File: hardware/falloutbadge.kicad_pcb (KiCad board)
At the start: 2 copper layers, 82 x 98.1 mm, 106 parts, among them J1 LiPo, J3 USB_C_Receptacle_USB2.0_16P, J4 E-INK, J5 Conn_01x03, Q2 NMOS, Q3 AO3400A, SW1 SW_Push, SW2 SW_Push, SW3 SW_Push, SW4 SW_Push, SW5 SW_Push, T1 BALFLB-WL-09D3, U1 CH592F, U2 STM32WLE5CCUx, U3 CH9102F, U4 USBLC6-2SC6, U5 TP4056, U6 BGS12SN6, U7 AP2112K-3.3, Y1 32MHz, Y2 32MHz

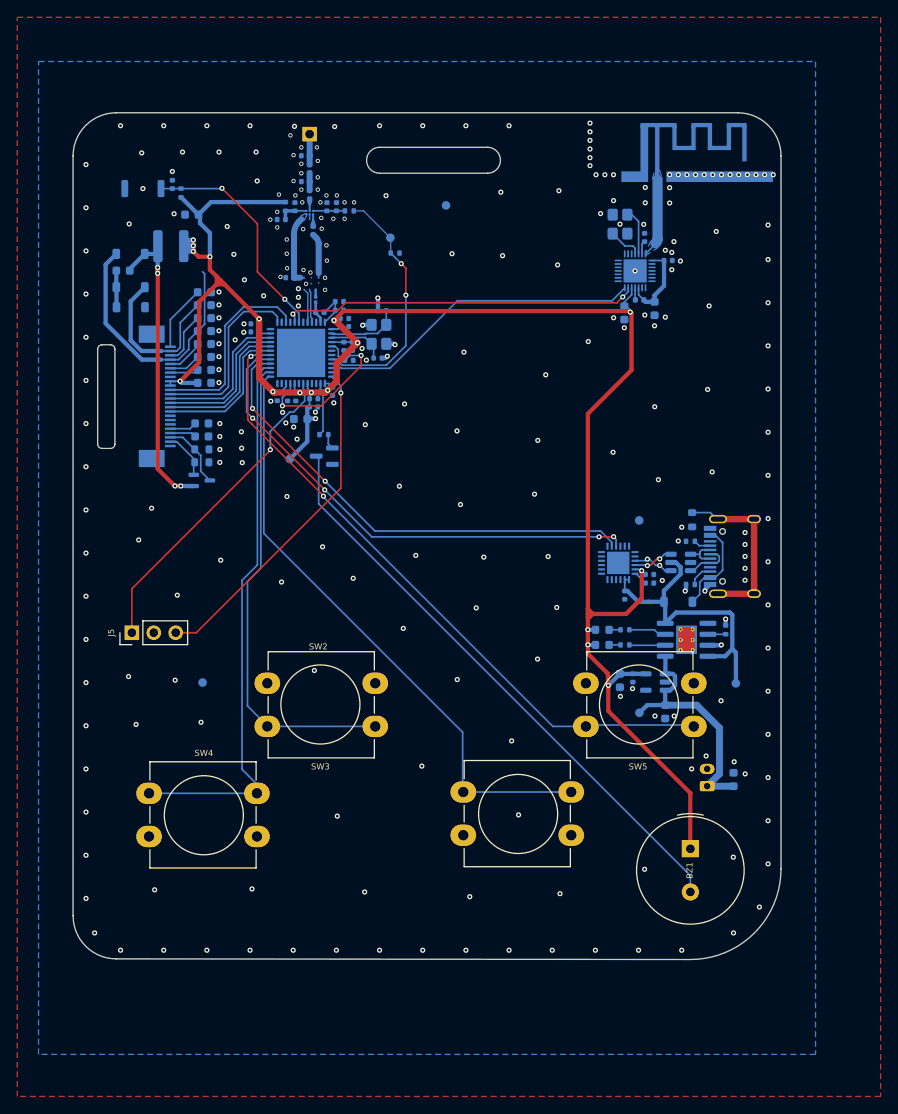
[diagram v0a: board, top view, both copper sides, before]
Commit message: final fixes
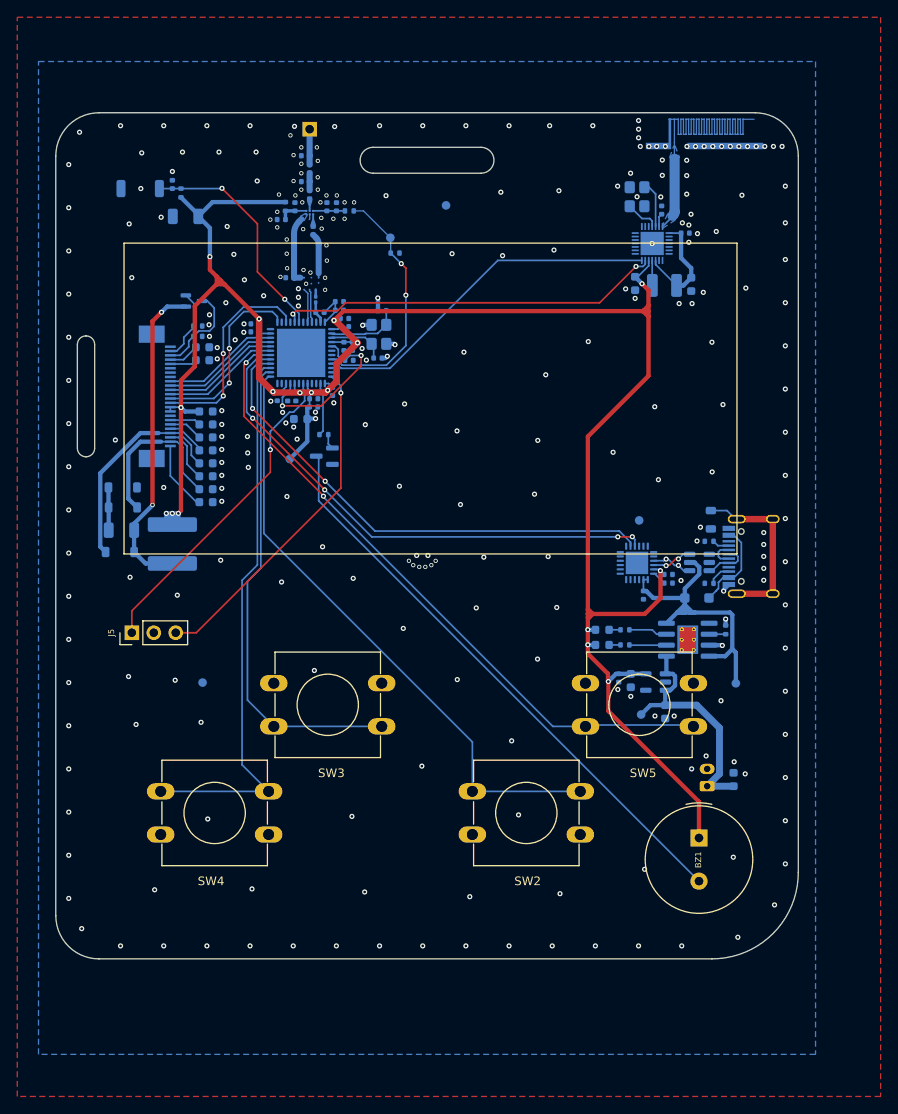
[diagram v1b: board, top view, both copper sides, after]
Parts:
- removed U5: TP4056, Package_SO:SOIC-8-1EP_3.9x4.9mm_P1.27mm_EP2.41x3.3mm_ThermalVias
- added U8: TP4056-42-ESOP8, Package_SO:SOIC-8-1EP_3.9x4.9mm_P1.27mm_EP2.41x3.3mm_ThermalVias, B.Cu at (176.3, 112.2)
- AE3: footprint antenna:ANT-F-1-2.4G-1.6mmFR4-WCH -> antenna:ANT-F-1-2.4G-0.8mmFR4-WCH
- C20, C22: footprint Capacitor_SMD:C_0603_1608Metric -> Capacitor_SMD:C_1206_3216Metric
- C42, C46: value 10uF -> 4.7uF
- C5, C6: value 20pF -> 6.8pF
- D1, D2, D3: value D -> MBR0530
- D4: footprint Diode_SMD:D_SOD-123 -> Diode_SMD:D_SOD-123F
- D8: value GREEN -> NOT RED
- FB1: footprint Resistor_SMD:R_0603_1608Metric -> Inductor_SMD:L_0805_2012Metric
- L1: value 47nH -> 68nH
- L3: footprint Inductor_SMD:L_APV_ANR4018 -> Inductor_SMD:L_Changjiang_FNR6028S
- L6: footprint Inductor_SMD:L_0402_1005Metric -> Inductor_SMD:L_1210_3225Metric
- Q2: value NMOS -> Si1308EDL
- R12, R13: value 1k -> 330R
- R6, R7: footprint Resistor_SMD:R_0603_1608Metric -> Resistor_SMD:R_0402_1005Metric
- SW1: footprint Button_Switch_SMD:SW_Push_SPST_NO_Alps_SKRK -> Button_Switch_SMD:SW_SPST_TS-1088-xR025
- SW2, SW3, SW4, SW5: footprint Button_Switch_THT:SW_PUSH-12mm_Wuerth-430476085716 -> Button_Switch_THT:SW_PUSH-12mm
- moved D3 34.5 mm to (110.6, 102.0)
- moved L3 34.5 mm to (116.7, 101.1), turned to -90 degrees
- moved C22 30.1 mm to (110.8, 99.5)
- moved D2 25.5 mm to (110.9, 96.8)
- moved C33 24.3 mm to (120.5, 96.2)
- moved C32 21.3 mm to (120.5, 94.7)
- moved D1 20.9 mm to (110.9, 94.5)
- moved Q2 20.8 mm to (119.2, 72.9)
- moved C31 18.3 mm to (120.5, 93.2)
- moved R6 15.8 mm to (119.6, 75.8)
- moved C30 15.3 mm to (120.5, 91.7)
- moved R7 13.1 mm to (119.6, 77.0)
- moved C29 12.3 mm to (120.5, 90.2)
- moved C25 10.3 mm to (120.2, 78.3)
- moved AE3 9.75 mm to (182.0, 54.5)
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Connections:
- C25 pad 2: Net-(J4-Pin_4) -> Net-(J4-Pin_21)
- C26 pad 2: Net-(J4-Pin_5) -> Net-(J4-Pin_20)
- C27 pad 2: Net-(J4-Pin_18) -> Net-(J4-Pin_7)
- C28 pad 2: Net-(J4-Pin_19) -> Net-(J4-Pin_6)
- C29 pad 2: Net-(J4-Pin_20) -> Net-(J4-Pin_5)
- C31 pad 2: Net-(J4-Pin_22) -> Net-(J4-Pin_3)
- C33 pad 2: Net-(J4-Pin_24) -> Net-(J4-Pin_1)
- J4 pad 1: unconnected-(J4-Pin_1-Pad1) -> Net-(J4-Pin_1)
- J4 pad 10: /RST -> +3V3
- J4 pad 11: /DC -> /SPI_MOSI
- J4 pad 12: /CS -> /SPI_SCK
- J4 pad 13: /SPI_SCK -> /CS
- J4 pad 14: /SPI_MOSI -> /DC
- J4 pad 15: +3V3 -> /RST
- J4 pad 16: +3V3 -> /BUSY
- J4 pad 18: Net-(J4-Pin_18) -> unconnected-(J4-Pin_18-Pad18)
- J4 pad 19: Net-(J4-Pin_19) -> unconnected-(J4-Pin_19-Pad19)
- J4 pad 2: /GDR -> /PREVGL
- J4 pad 21: /PREVGH -> Net-(J4-Pin_21)
- J4 pad 22: Net-(J4-Pin_22) -> /RESE
- J4 pad 23: /PREVGL -> /GDR
- J4 pad 24: Net-(J4-Pin_24) -> unconnected-(J4-Pin_24-Pad24)
- J4 pad 3: /RESE -> Net-(J4-Pin_3)
- J4 pad 4: Net-(J4-Pin_4) -> /PREVGH
- J4 pad 6: unconnected-(J4-Pin_6-Pad6) -> Net-(J4-Pin_6)
- J4 pad 7: unconnected-(J4-Pin_7-Pad7) -> Net-(J4-Pin_7)
- J4 pad 9: /BUSY -> +3V3
- U2 pad 10: /CS -> /BUSY
- U2 pad 7: /BUSY -> /CS
- U2 pad 8: /RST -> /DC
- U2 pad 9: /DC -> /RST
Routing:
- net +3V3: track 237.8 -> 261.0 mm
- net Net-(J4-Pin_1): track 0.00 -> 8.09 mm
- net Net-(J4-Pin_24): track 7.90 -> 0.00 mm
- net Net-(J4-Pin_3): track 0.00 -> 6.45 mm
- net Net-(J4-Pin_22): track 6.13 -> 0.00 mm
- net /PREVGH: track 30.3 -> 24.9 mm
- net Net-(J4-Pin_6): track 0.00 -> 3.98 mm
- net Net-(J4-Pin_19): track 3.71 -> 0.00 mm
- net Net-(J4-Pin_7): track 0.00 -> 3.57 mm
- net Net-(J4-Pin_21): track 0.00 -> 3.55 mm
- net VBUS: track 35.2 -> 38.7 mm
- net /VDCIA: track 9.62 -> 13.0 mm
- net /CS: track 17.0 -> 13.7 mm
- net /UART1_TX: track 38.0 -> 41.3 mm
- net Net-(J4-Pin_18): track 3.30 -> 0.00 mm
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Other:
- board size 82 x 98.1 mm -> 86 x 98 mm
